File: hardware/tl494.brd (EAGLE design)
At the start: 100 x 80 mm, 85 parts, among them IC1 TL494CN, J1 CON_HEADER_1X02-PTH, J2 CON_HEADER_1X02-PTH, K2 24V, Q1 2N5551, Q1I 8050, Q1I1 2N3904, Q2 8550, Q2I 8050, Q3 8050, Q4 2SK4145, Q6 IRF9540, T1 PAD_TERMINAL-1.02MM_ROUND, T2 PAD_TERMINAL-1.02MM_ROUND, T3 PAD_TERMINAL-1.02MM_SQUARE, T4 PAD_TERMINAL-1.02MM_ROUND

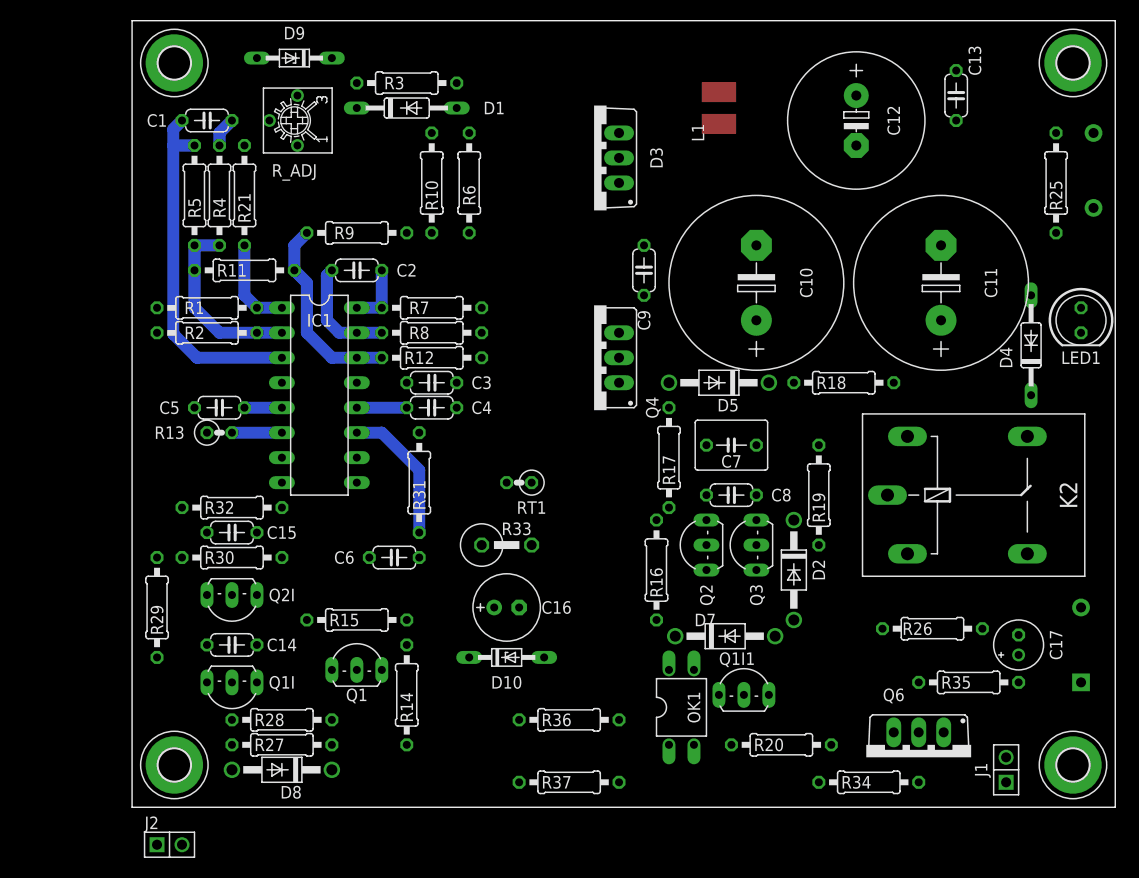
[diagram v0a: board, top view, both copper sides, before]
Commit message: done board routing
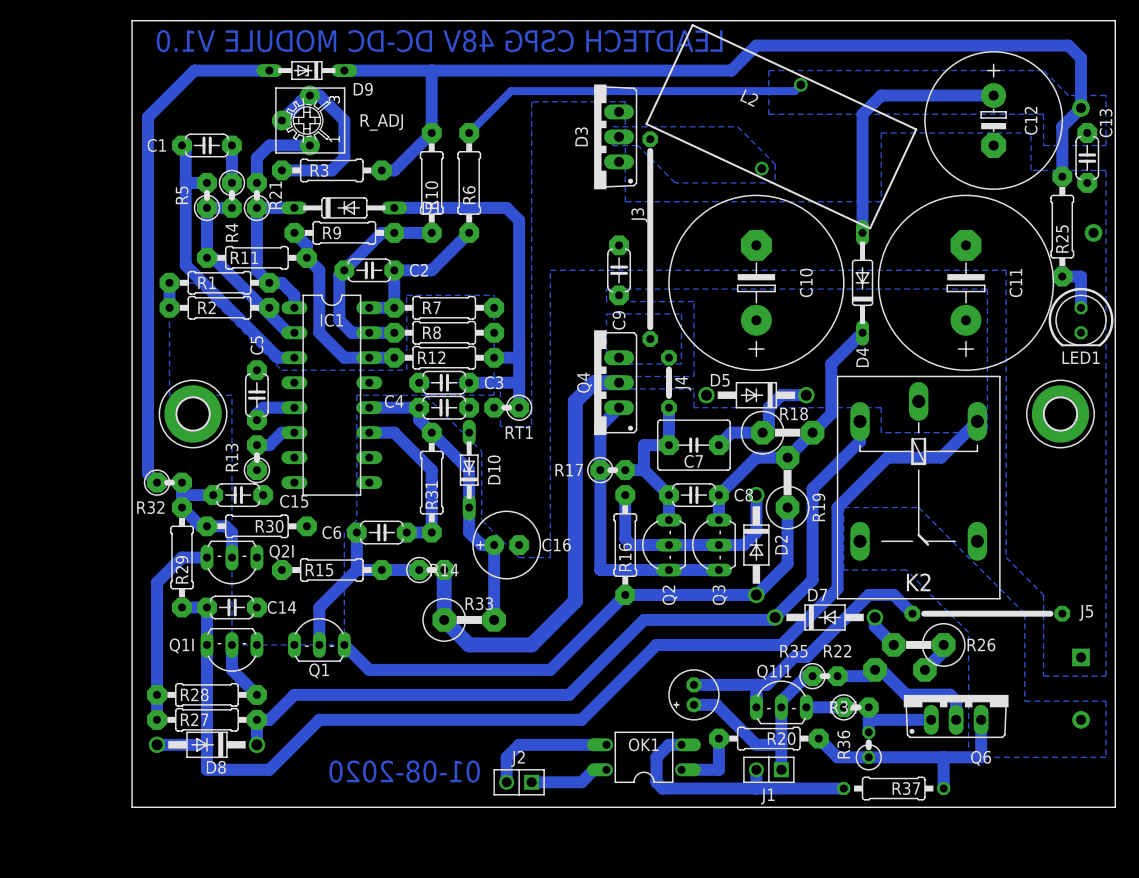
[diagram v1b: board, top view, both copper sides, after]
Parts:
- removed H3, H4: MOUNT-PAD-ROUND3.3, holes:3,3-PAD
- removed L1: INDUCTOR-L1812, dp_devices.v6:L1812
- added J3: J20MM, jumper:20
- added J4: J5MM, jumper:05
- added J5: J15MM, jumper:15
- added L2: (no value), rcl:TJ5-U1
- added R22: 560R 1W, trosh_devices.eagle.v9:0414V_EXPAD
- C1, C13, C14, C15, C2, C3, C4, C5, C6, C8, C9: device rcl:C050-024X044 -> trosh_devices.eagle.v9:C050-024X044_EXPAD
- C16: device rcl:E2,5-7 -> trosh_devices.eagle.v9:E2,5-7_EXPAD
- C17: device rcl:E2-5 -> trosh_devices.eagle.v9:E2-5_EXPAD
- C7: device rcl:C050-050X075 -> trosh_devices.eagle.v9:C050-050X075_EXPAD
- R1, R10, R11, R12, R15, R16, R2, R20, R25, R27, R28, R29, R3, R30, R31, R6, R7, R8, R9: device rcl:0207/10 -> trosh_devices.eagle.v9:0207/10_EXPAD
- R13: device rcl:0207/2V -> trosh_devices.eagle.v9:0207/2V_EXPAD
- R14, R17, R21, R32, R34, R35, R4, R5: device rcl:0207/10 -> trosh_devices.eagle.v9:0207/2V_EXPAD
- R18, R19: device rcl:0207/10 -> trosh_devices.eagle.v9:0414V_EXPAD
- R26: value 560*x2 1W -> 560R 1W; device rcl:0207/10 -> trosh_devices.eagle.v9:0414V_EXPAD
- R33: device rcl:0414V -> trosh_devices.eagle.v9:0414V_EXPAD
- R36: device rcl:0207/10 -> rcl:0207/2V
- RT1: value (none) -> RESISTOR0207/2V_EXPAD; device rcl:0207/2V -> trosh_devices.eagle.v9:0207/2V_EXPAD
- R_ADJ: device dp_devices.v6:TRIMMER_3362P -> trosh_devices.eagle.v9:TRIMMER_3362P_EXPAD
- moved H1 96.9 mm to (94.4, 40.0)
- moved J2 36.1 mm to (39.4, 2.54), turned to 180 degrees
- moved H2 35.8 mm to (6.21, 40.0)
- moved C17 33.4 mm to (57.1, 11.4)
- moved R37 33.0 mm to (77.5, 1.91), turned to 180 degrees
- moved R36 30.6 mm to (74.9, 6.35), turned to 90 degrees
- moved J1 24.1 mm to (64.8, 3.81), turned to 180 degrees
- moved D10 19.4 mm to (34.3, 34.3), turned to 90 degrees
- moved D4 18.3 mm to (74.3, 53.3)
- moved C13 14.8 mm to (97.2, 66.0)
- moved R35 14.6 mm to (70.5, 13.3), turned to 0 degrees
- moved C12 14.0 mm to (87.6, 69.8)
- moved R14 13.0 mm to (30.5, 24.1), turned to 0 degrees
- moved D1 12.0 mm to (21.6, 61.0)
- moved R3 11.7 mm to (20.3, 64.8)
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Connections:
- new net N$36: R22.2, R26.1
- new net N$37: D3.C, J3.2, L2.2
- new net N$38: J3.1, J4.1, Q4.3
- net +15V: now also R33.2; no longer R33.1
- net +V: now also R33.1; no longer R33.2
- net GND: now also J5.1, J5.2
- net N$17: now also J4.2; no longer D3.C, L1.1, Q4.3
- net N$18: now also R18.2; no longer R18.1
- net N$19: now also R18.1; no longer R18.2
- net N$22: now also R26.2; no longer R26.1
- net N$32: now also R22.1; no longer R26.2
- net VOUT: now also L2.1; no longer L1.2
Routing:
- net VOUT: track 0.00 -> 164.3 mm
- net N$24: track 0.00 -> 122.0 mm
- net N$23: track 0.00 -> 83.1 mm
- net N$14: track 0.00 -> 56.3 mm
- net N$28: track 0.00 -> 51.9 mm
- net +V: track 0.00 -> 46.9 mm
- net N$9: track 0.00 -> 39.9 mm
- net GND: track 0.00 -> 32.9 mm
- net N$16: track 0.00 -> 29.4 mm
- net N$18: track 0.00 -> 27.0 mm
- net N$34: track 0.00 -> 26.8 mm
- net +15V: track 5.08 -> 30.6 mm
- net VIN: track 0.00 -> 24.3 mm
- net N$15: track 0.00 -> 22.4 mm
- net N$33: track 0.00 -> 21.8 mm
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- added copper zone on layer 16, net +V
- added copper zone on layer 16, net GND
- added copper zone on layer 16, net N$37
- added copper zone on layer 16, net N$38
- added copper zone on layer 16, net VIN
- added copper zone on layer 16, net VOUT
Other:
- board text added: "01-08-2020"
- board text added: "LEADTECH CSPG 48V DC-DC MODULE V1.0"
